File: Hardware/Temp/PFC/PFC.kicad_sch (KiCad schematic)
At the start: 9 parts, among them J1 HB9500M-9.5-3P, U1 UCC28180D

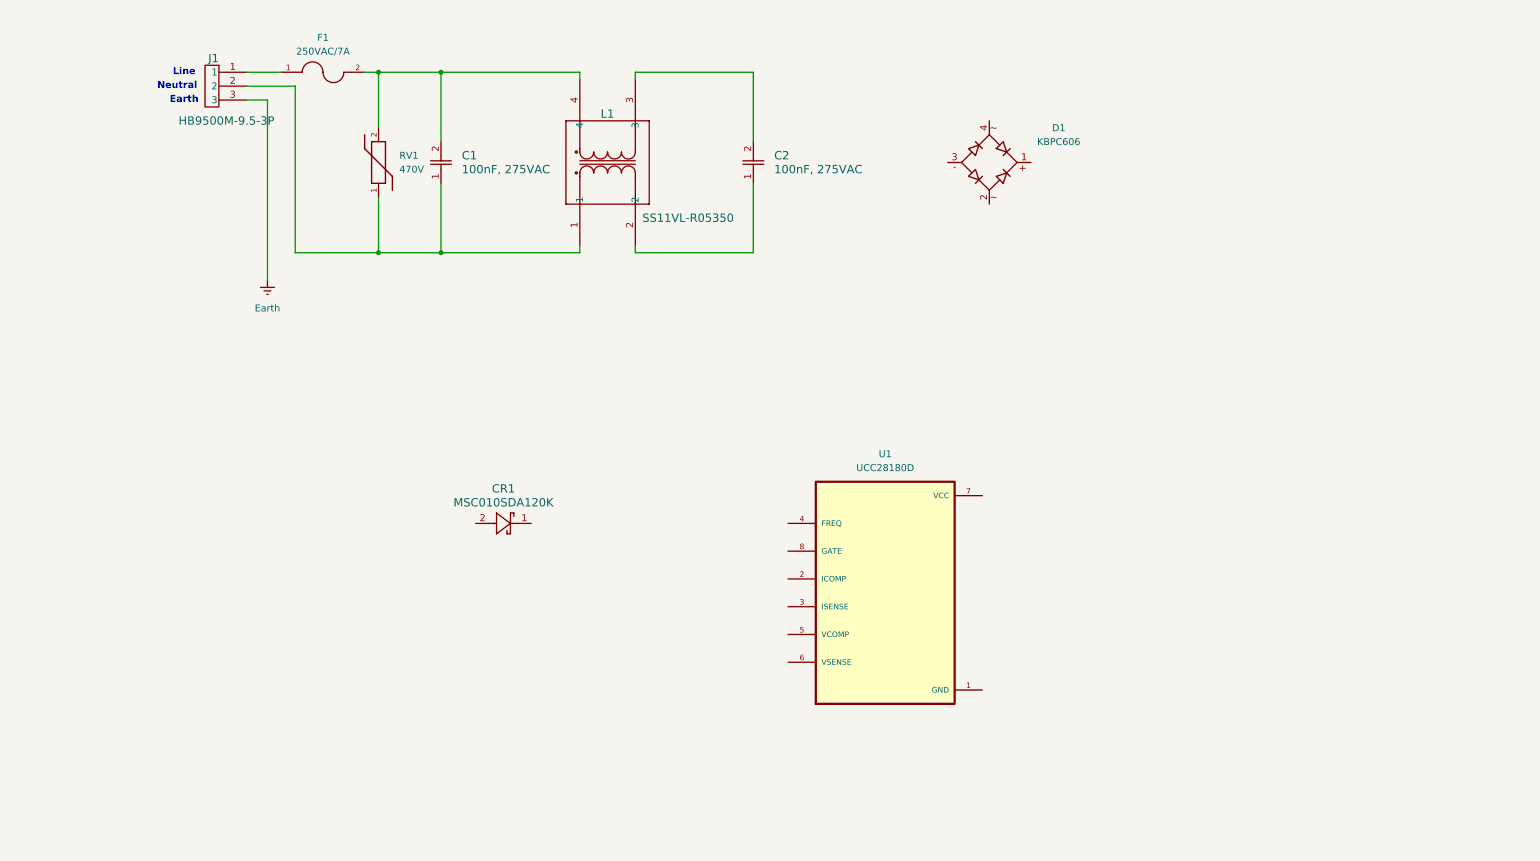
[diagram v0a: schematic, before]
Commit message: change schematic
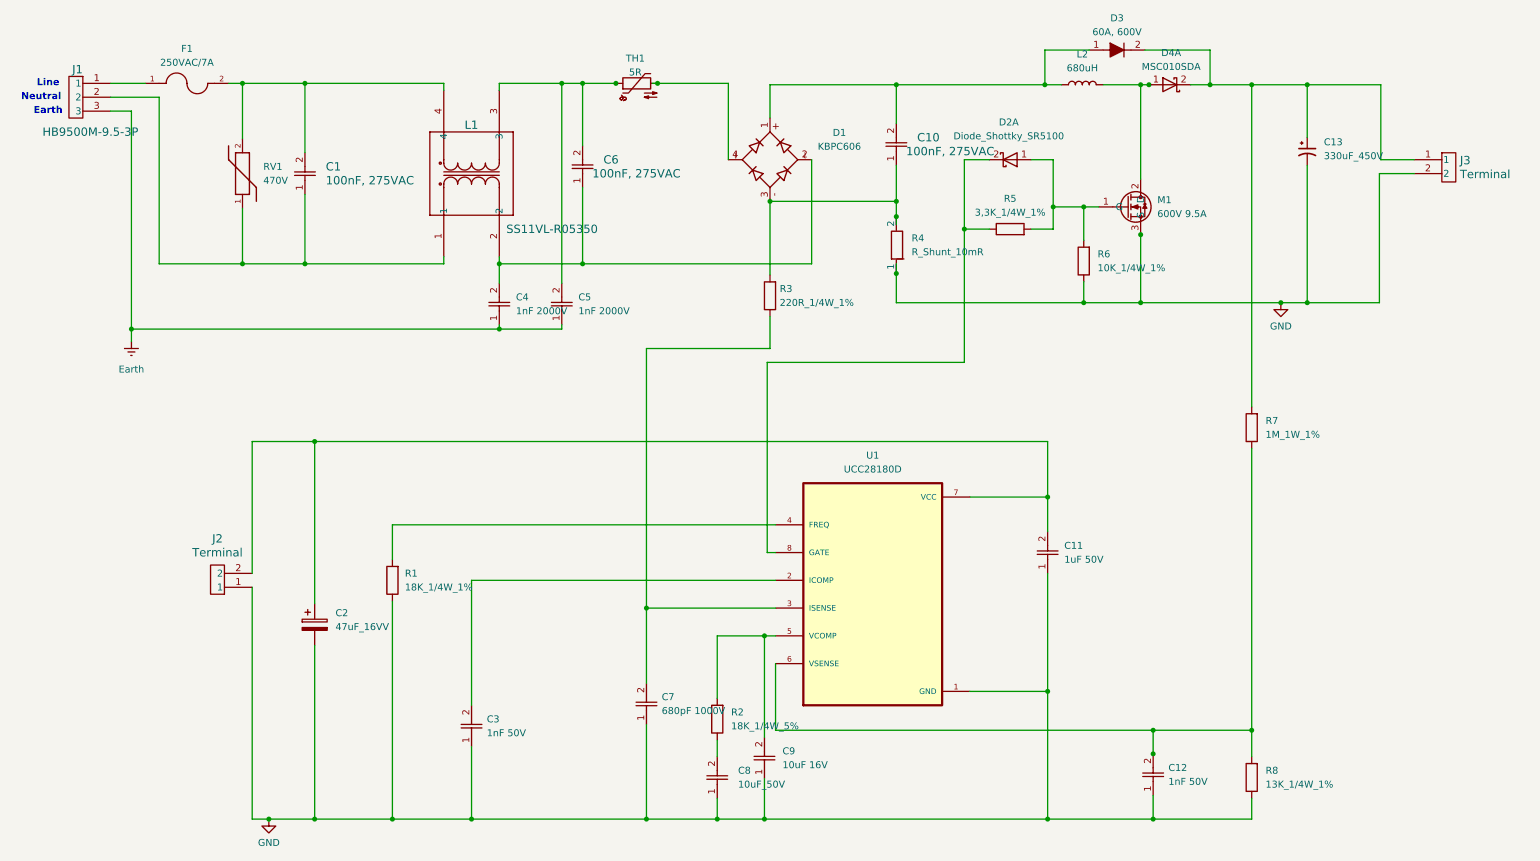
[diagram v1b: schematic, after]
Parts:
- removed C2: 100nF, 275VAC, charge_battery_footprint_lib:CAP_B32671P-10--5x11x13_TDK, symbol charge_battery_sym_lib:Film Cap
- removed CR1: MSC010SDA120K, charge_battery_footprint_lib:TO-220-2_MCH, symbol charge_battery_sym_lib:MSC010SDA120K
- added C10, C6: 100nF, 275VAC, charge_battery_footprint_lib:CAP_B32671P-10--5x11x13_TDK, symbol charge_battery_sym_lib:Film Cap
- added C11: 1uF 50V, charge_battery_footprint_lib:Ceramic_Cap_Hole_1uF_50V, symbol charge_battery_sym_lib:Ceramic_Cap_Hole_1uF_50V_
- added C12, C3: 1nF 50V, charge_battery_footprint_lib:Ceramic_Cap_Hole_1nF_50V, symbol charge_battery_sym_lib:Ceramic_Cap_Hole_1nF_50V
- added C13: 330uF_450V, charge_battery_footprint_lib:Big_Cap_330uF_450V, symbol charge_battery_sym_lib:Cap_Polarized_330uF_450V
- added C2: 47uF_16VV, charge_battery_footprint_lib:Cap_Polarized_SMD_47uF_16V, symbol charge_battery_sym_lib:Cap_Polarized_SMD_47uF_16V
- added C4, C5: 1nF 2000V, charge_battery_footprint_lib:Ceramic_Cap_Hole_1nF_2000V, symbol charge_battery_sym_lib:Ceramic_Cap_Hole_680pF_1000V
- added C7: 680pF 1000V, charge_battery_footprint_lib:Ceramic_Cap_Hole_680pF_1000V, symbol charge_battery_sym_lib:Ceramic_Cap_Hole_1nF_2000V
- added C8: 10uF_50V, Capacitor_SMD:C_0805_2012Metric, symbol charge_battery_sym_lib:Ceramic_Cap_Hole_10uF_50V
- added C9: 10uF 16V, charge_battery_footprint_lib:Ceramic_Cap_10uF_16V, symbol charge_battery_sym_lib:Ceramic_Cap_SMD_10uF_16V
- added D2: Diode_Shottky_SR5100, charge_battery_footprint_lib:Diode_Schottky_SR5100, symbol charge_battery_sym_lib:Diode_Shottky_SR5100
- added D3: 60A, 600V, charge_battery_footprint_lib:Diode_FRED_TO247, symbol charge_battery_sym_lib:Diode_DSEI60-06A_FRED_TO247
- added D4: MSC010SDA, charge_battery_footprint_lib:DBoost, symbol charge_battery_sym_lib:Diode_Shottky_DBoost
- added J2, J3: Terminal, charge_battery_footprint_lib:Terminal, symbol charge_battery_sym_lib:Terminal HB9500-2
- added L2: 680uH, Inductor_SMD:L_12x12mm_H8mm, symbol Device:L
- added M1: 600V 9.5A, charge_battery_footprint_lib:MOSFET_FQPF10N60C, symbol charge_battery_sym_lib:MOSFET_FQPF10N60C
- added R1: 18K_1/4W_1%, charge_battery_footprint_lib:Res_220R_1_4W_1%, symbol charge_battery_sym_lib:Res_hole_18K_1/4W_1%
- added R2: 18K_1/4W_5%, charge_battery_footprint_lib:Res_220R_1_4W_1%, symbol charge_battery_sym_lib:Res_hole_18K_1/4W_1%
- added R3: 220R_1/4W_1%, charge_battery_footprint_lib:Res_220R_1_4W_1%, symbol charge_battery_sym_lib:Res_hole_220R_1/4W_1%
- added R4: R_Shunt_10mR, charge_battery_footprint_lib:R_Shunt, symbol charge_battery_sym_lib:R_Shunt_10mR
- added R5: 3,3K_1/4W_1%, charge_battery_footprint_lib:Res_3.3R_1_4W_1, symbol charge_battery_sym_lib:Res_hole_3,3K_1/4W_1%
- added R6: 10K_1/4W_1%, charge_battery_footprint_lib:Res_10K_1_4W_1%, symbol charge_battery_sym_lib:Res_hole_10K_1/4W_1%
- added R7: 1M_1W_1%, charge_battery_footprint_lib:Res_1M_1W_1%, symbol charge_battery_sym_lib:Res_hole_1M_1W_1%
- added R8: 13K_1/4W_1%, charge_battery_footprint_lib:Res_13K_1_4W_1, symbol charge_battery_sym_lib:Res_hole_13K_1/4W_1%
- added TH1: 5R, charge_battery_footprint_lib:Thermistor_NTC, symbol charge_battery_sym_lib:Thermistor_NTC
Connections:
- net Earth: now also C4.1, C5.1
- net at L1.2: now also D1.2, C4.2, C6.1
- net at L1.3: now also C5.2, C6.2, TH1.1
- net GND: now reaches U1.1 (GND)
- net GND: now also C11.1, C12.1, C13.2, C2.2, C3.1, C7.1, C8.1, C9.1, J2.1, J3.2, M1.3 (S), R1.1, R4.1, R6.1, R8.1
- net at U1.2 (ICOMP): now also C3.2
- net at U1.3 (ISENSE): now also C7.2, R3.1
- net at U1.4 (FREQ): now also R1.2
- net at U1.5 (VCOMP): now also C9.2, R2.2
- net at U1.6 (VSENSE): now also C12.2, R7.1, R8.2
- net at U1.7 (VCC): now also C11.2, C2.1, J2.2
- net at U1.8 (GATE): now also D2.2 (A), R5.1
- net at D1.1: now also C10.2, D3.1, L2.1
- net at D1.3: now also C10.1, R3.2, R4.2
- net at D1.4: now also TH1.2
- new net: D2.1 (K), M1.1 (G), R5.2, R6.2
- new net: C13.1, D3.2, D4.2 (A), J3.1, R7.2
- new net: D4.1 (K), L2.2, M1.2 (D)
- new net: C8.2, R2.1
